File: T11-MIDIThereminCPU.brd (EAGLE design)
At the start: 103.8 x 81.3 mm, 62 parts, among them IC1 UA78M05DCY, IC4 QUAD_OPAMPD, IC5 4069D, J1 DCJ0202, Q1 16MHz, U1 ATMEGA328P-AU

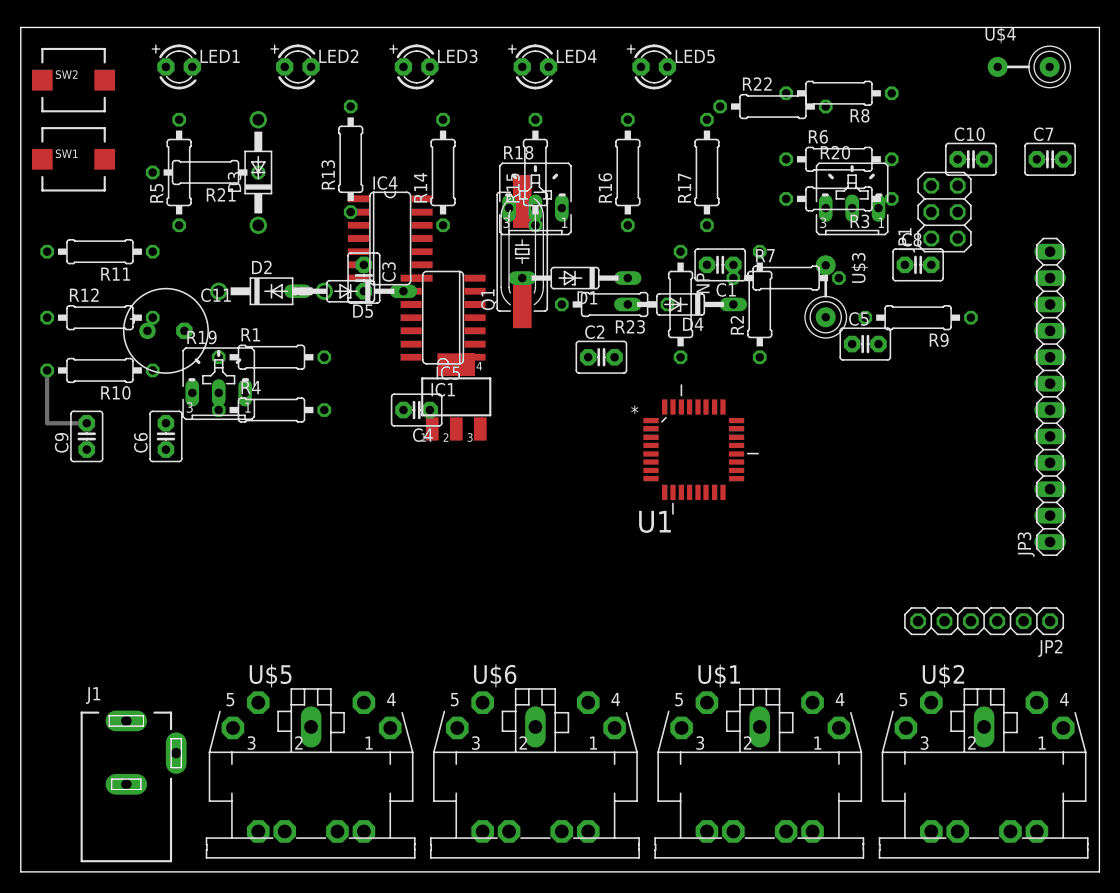
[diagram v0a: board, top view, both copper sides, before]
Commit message: Board creation
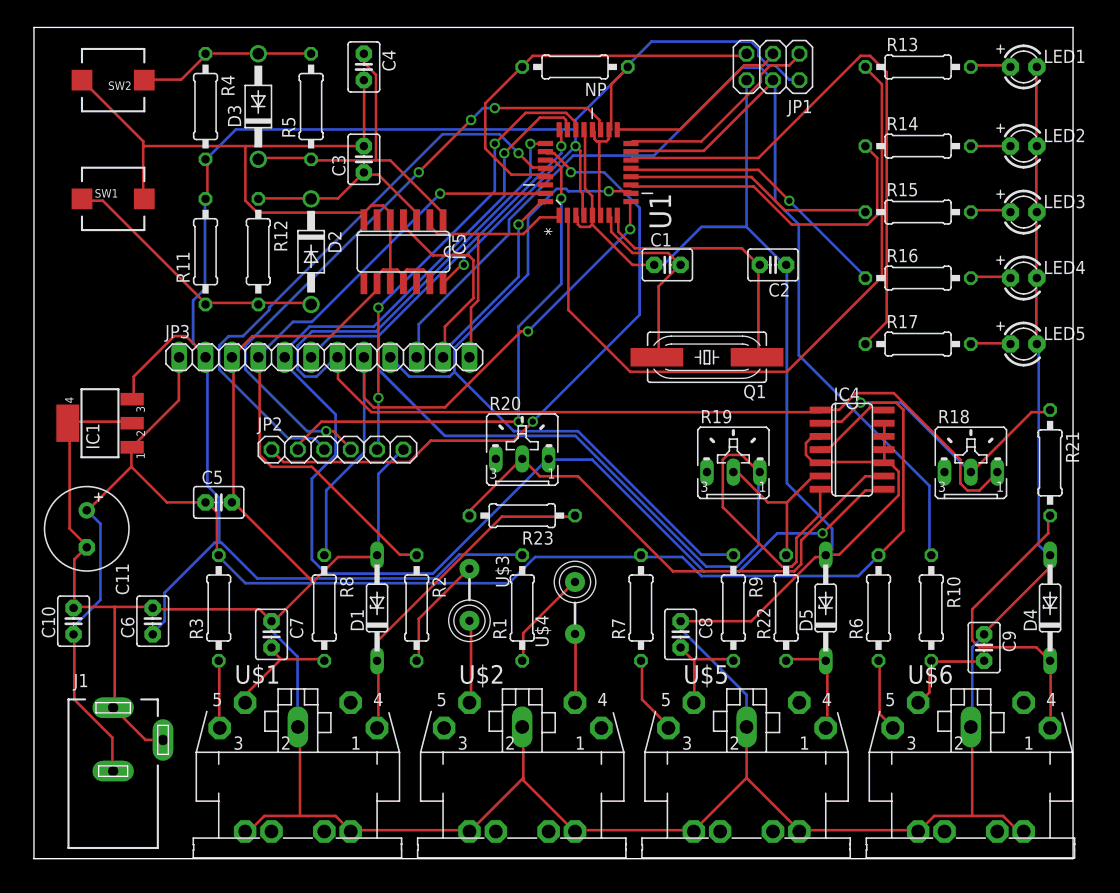
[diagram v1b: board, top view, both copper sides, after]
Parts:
- moved C10 97.1 mm to (3.81, 22.9), turned to 90 degrees
- moved C9 88.7 mm to (91.4, 20.3), turned to 270 degrees
- moved C7 87.8 mm to (22.9, 21.6), turned to 270 degrees
- moved R21 85.9 mm to (97.8, 38.1), turned to 270 degrees
- moved R10 83.2 mm to (86.4, 24.1), turned to 270 degrees
- moved LED1 81.3 mm to (95.2, 76.2)
- moved R3 71.5 mm to (17.8, 24.1), turned to 90 degrees
- moved LED2 70.3 mm to (95.2, 68.6)
- moved R8 70.0 mm to (27.9, 24.1), turned to 270 degrees
- moved JP3 70.0 mm to (27.9, 48.3), turned to 0 degrees
- moved U$4 67.6 mm to (52.1, 24.1), turned to 90 degrees
- moved JP2 64.4 mm to (29.2, 39.4), turned to 0 degrees
- moved C5 64.1 mm to (17.8, 34.3)
- moved LED3 60.1 mm to (95.2, 62.2)
- moved R13 55.3 mm to (85.1, 76.2), turned to 0 degrees
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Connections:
- net GND: now also IC4.12, IC4.13, IC5.11, IC5.13, IC5.5, IC5.9
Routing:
- net GND: track 0.00 -> 535.0 mm
- net +5V: track 0.00 -> 202.9 mm, vias 0 -> 2
- net +12V: track 0.00 -> 154.0 mm
- net ANALOG_IN_1: track 0.00 -> 130.9 mm, vias 0 -> 2
- net MOSI: track 0.00 -> 117.6 mm
- net ANALOG_IN_2: track 0.00 -> 116.7 mm, vias 0 -> 1
- net ANALOG_IN_3: track 0.00 -> 114.7 mm, vias 0 -> 1
- net SIGNAL_OUT_2: track 0.00 -> 70.4 mm, vias 0 -> 1
- net LED_1: track 0.00 -> 66.4 mm
- net PC3: track 0.00 -> 63.6 mm, vias 0 -> 2
- net TX: track 0.00 -> 62.8 mm, vias 0 -> 1
- net ADC6: track 0.00 -> 60.7 mm, vias 0 -> 4
- net SIGNAL_OUT_1: track 0.00 -> 60.4 mm, vias 0 -> 2
- net PC5: track 0.00 -> 57.0 mm, vias 0 -> 1
- net LED_5: track 0.00 -> 56.4 mm
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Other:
- board size 103.8 x 81.3 mm -> 100 x 80 mm
